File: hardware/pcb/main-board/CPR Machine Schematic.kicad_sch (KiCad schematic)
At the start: 0 parts

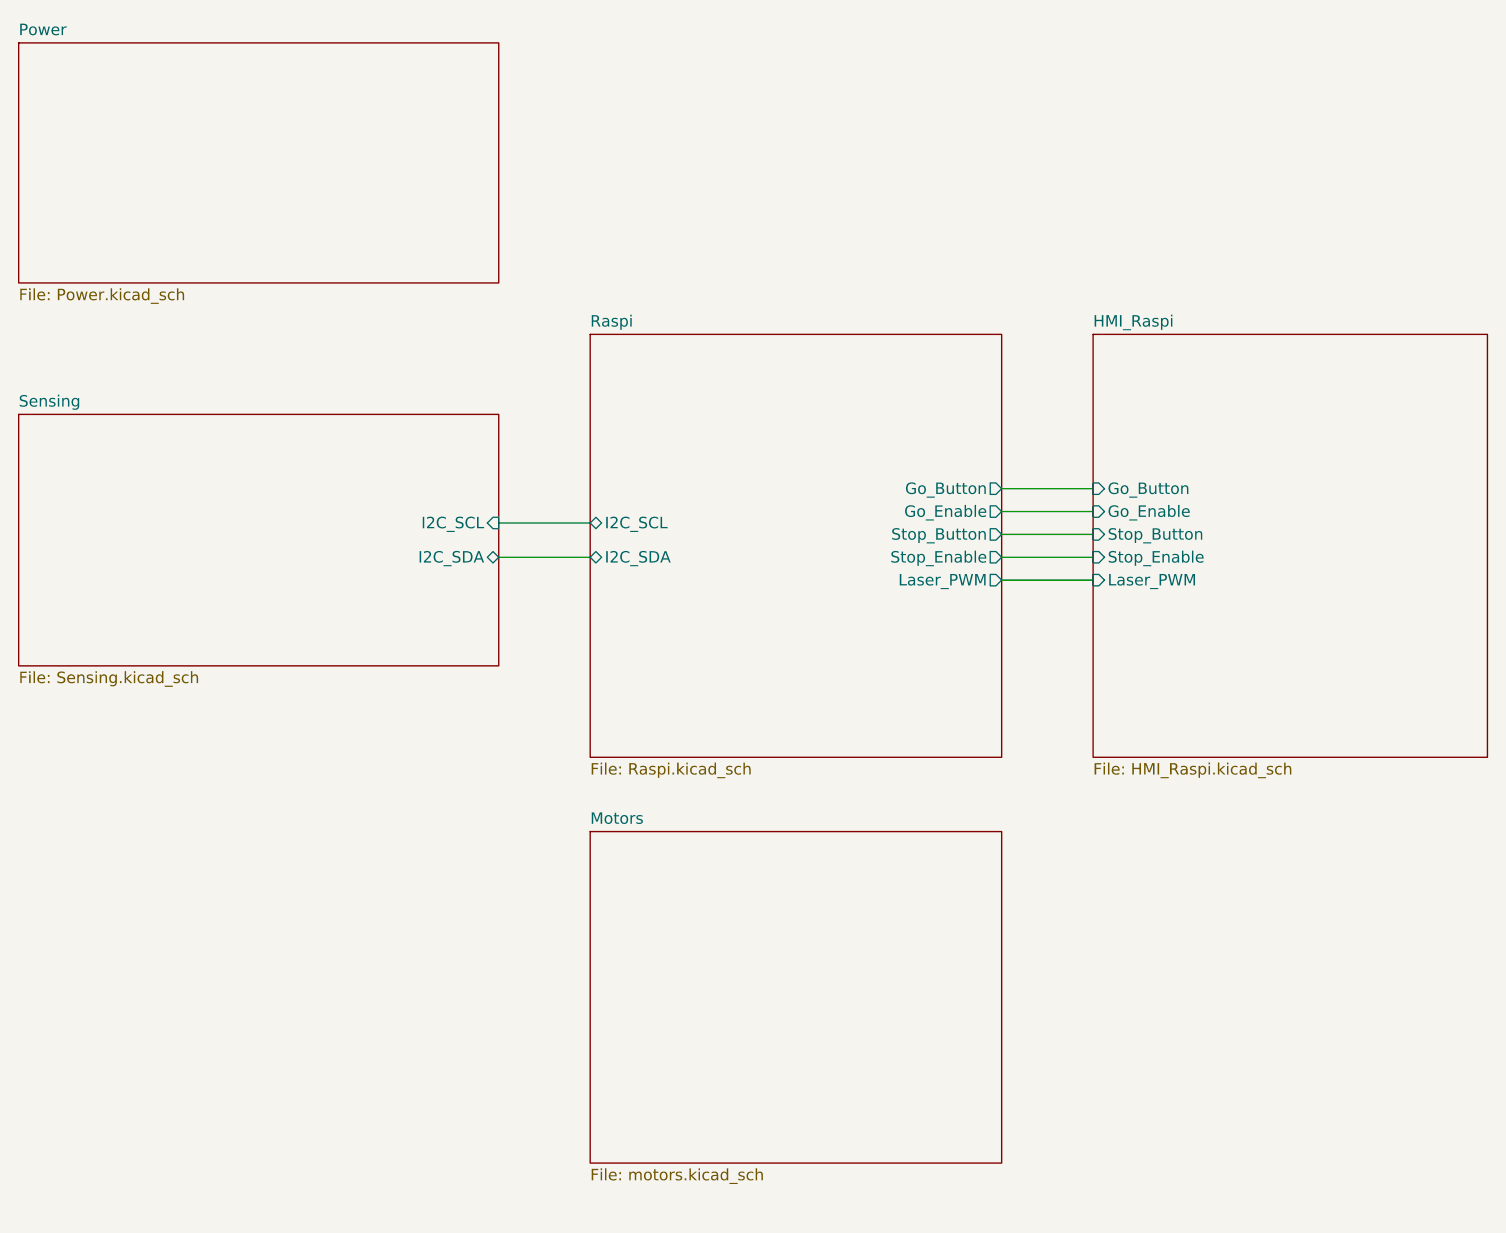
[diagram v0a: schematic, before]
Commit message: Start of CAN-FD
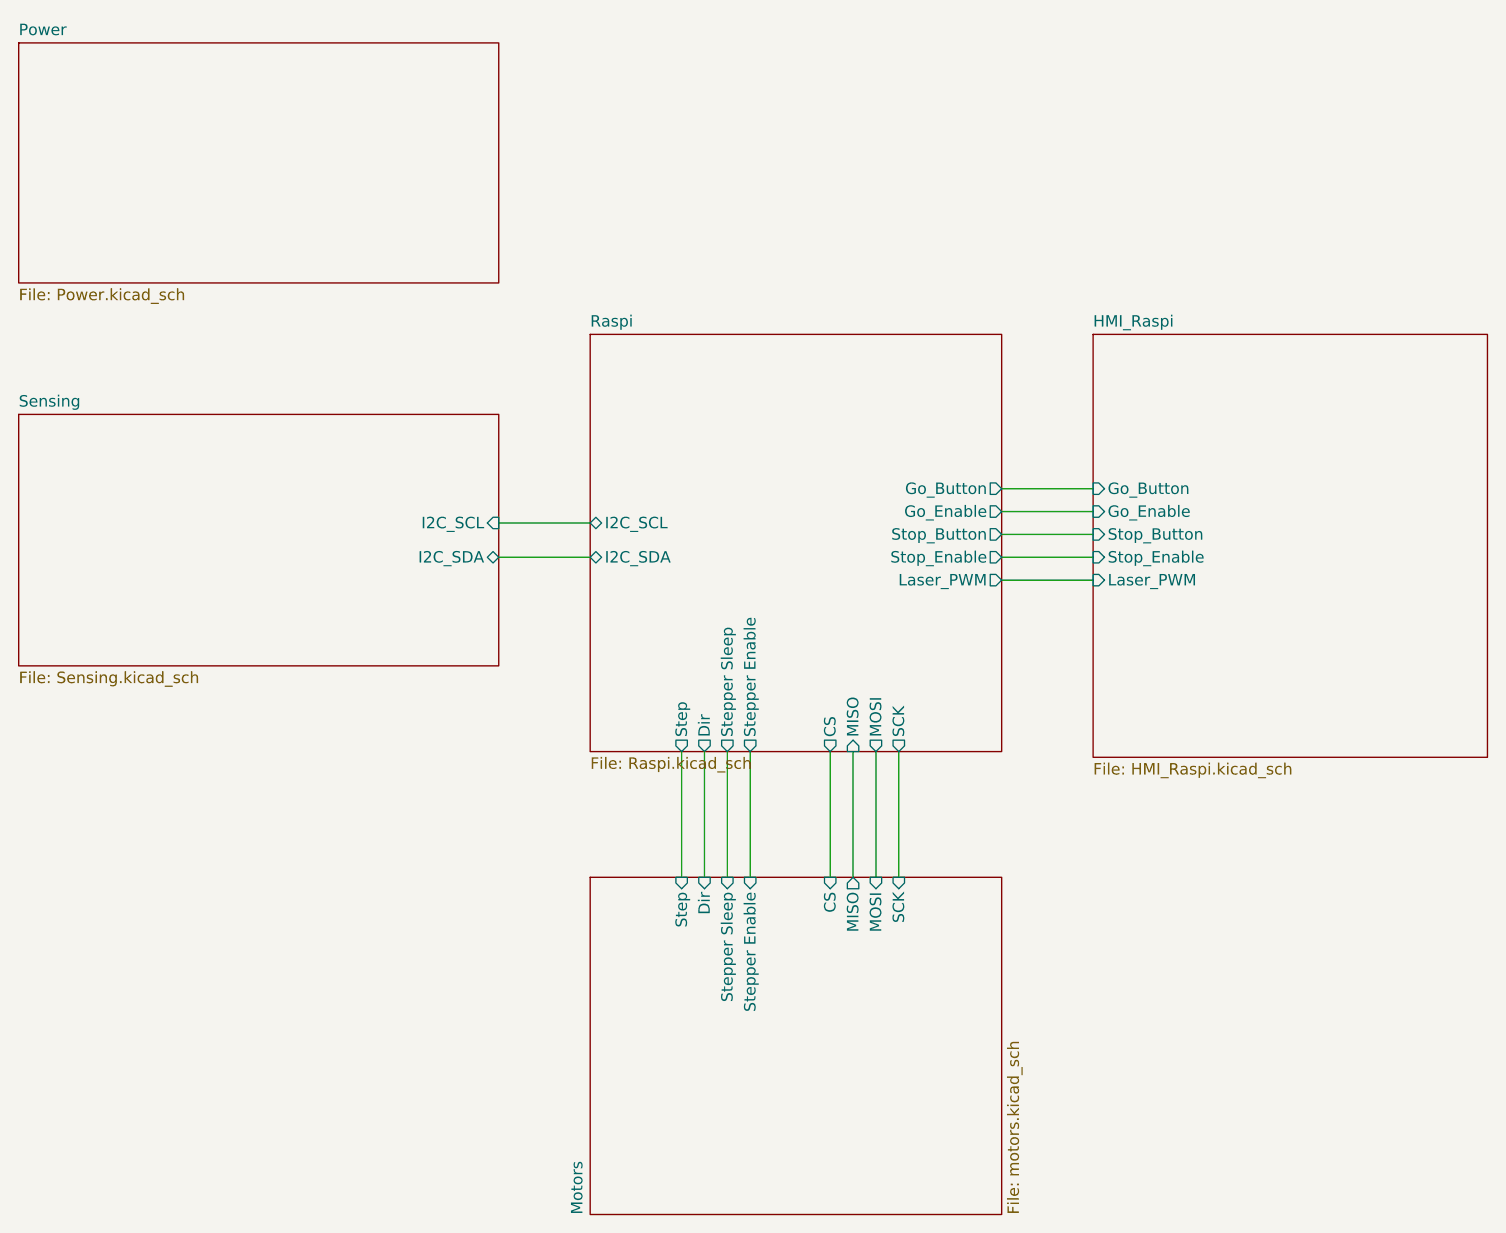
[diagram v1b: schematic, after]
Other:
- sheet Motors ports: added CS, Dir, MISO, MOSI, SCK, Step, Stepper Enable, Stepper Sleep; removed none
- sheet Raspi ports: added CS, Dir, MISO, MOSI, SCK, Step, Stepper Enable, Stepper Sleep; removed none
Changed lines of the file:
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@@
+	(wire
+		(pts
+			(xy 138.43 105.41) (xy 138.43 119.38)
+		)
+		(stroke
+			(width 0)
+			(type default)
+		)
+	)
 	(wire
 		(pts
@@
 	(wire
 		(pts
+			(xy 133.35 105.41) (xy 133.35 119.38)
+		)
+		(stroke
+			(width 0)
+			(type default)
+		)
+	)
+	(wire
+		(pts
+			(xy 130.81 105.41) (xy 130.81 119.38)
+		)
+		(stroke
+			(width 0)
+			(type default)
+		)
+	)
+	(wire
+		(pts
+			(xy 152.4 105.41) (xy 152.4 119.38)
+		)
+		(stroke
+			(width 0)
+			(type default)
+		)
+	)
+	(wire
+		(pts
+			(xy 147.32 105.41) (xy 147.32 119.38)
+		)
+		(stroke
+			(width 0)
+			(type default)
+		)
+	)
+	(wire
+		(pts
+			(xy 135.89 105.41) (xy 135.89 119.38)
+		)
+		(stroke
+			(width 0)
+			(type default)
+		)
+	)
+	(wire
+		(pts
 			(xy 166.37 83.82) (xy 176.53 83.82)
 		)
@@
 	(wire
 		(pts
+			(xy 154.94 105.41) (xy 154.94 119.38)
+		)
+		(stroke
+			(width 0)
+			(type default)
+		)
+	)
+	(wire
+		(pts
 			(xy 110.49 80.01) (xy 120.65 80.01)
 		)
@@
 		(pts
 			(xy 166.37 78.74) (xy 176.53 78.74)
+		)
+		(stroke
+			(width 0)
+			(type default)
+		)
+	)
+	(wire
+		(pts
+			(xy 149.86 105.41) (xy 149.86 119.38)
 		)
 		(stroke
@@
 	(sheet
 		(at 120.65 59.055)
-		(size 45.72 46.99)
+		(size 45.72 46.355)
 		(exclude_from_sim no)
 		(in_bom yes)
@@
 		)
 		(property "Sheetfile" "Raspi.kicad_sch"
-			(at 120.65 106.6296 0)
+			(at 120.65 105.9946 0)
 			(show_name no)
 			(do_not_autoplace no)
@@
 				)
 				(justify right)
+			)
+		)
+		(pin "Dir" output
+			(at 133.35 105.41 270)
+			(effects
+				(font
+					(size 1.27 1.27)
+				)
+				(justify left)
+			)
+		)
+		(pin "Step" output
+			(at 130.81 105.41 270)
+			(effects
+				(font
+					(size 1.27 1.27)
+				)
+				(justify left)
+			)
+		)
+		(pin "Stepper Enable" output
+			(at 138.43 105.41 270)
+			(effects
+				(font
+					(size 1.27 1.27)
+				)
+				(justify left)
+			)
+		)
+		(pin "Stepper Sleep" output
+			(at 135.89 105.41 270)
+			(effects
+				(font
+					(size 1.27 1.27)
+				)
+				(justify left)
+			)
+		)
+		(pin "MISO" input
+			(at 149.86 105.41 270)
+			(effects
+				(font
+					(size 1.27 1.27)
+				)
+				(justify left)
+			)
+		)
+		(pin "MOSI" output
+			(at 152.4 105.41 270)
+			(effects
+				(font
+					(size 1.27 1.27)
+				)
+				(justify left)
+			)
+		)
+		(pin "SCK" output
+			(at 154.94 105.41 270)
+			(effects
+				(font
+					(size 1.27 1.27)
+				)
+				(justify left)
+			)
+		)
+		(pin "CS" output
+			(at 147.32 105.41 270)
+			(effects
+				(font
+					(size 1.27 1.27)
+				)
+				(justify left)
 			)
 		)
@@
 	)
 	(sheet
-		(at 120.65 114.3)
-		(size 45.72 36.83)
+		(at 120.65 119.38)
+		(size 45.72 37.465)
 		(exclude_from_sim no)
 		(in_bom yes)
@@
 		)
 		(property "Sheetname" "Motors"
-			(at 120.65 113.5884 0)
+			(at 119.9384 156.845 90)
 			(show_name no)
 			(do_not_autoplace no)
@@
 		)
 		(property "Sheetfile" "motors.kicad_sch"
-			(at 120.65 151.7146 0)
+			(at 166.9546 156.845 90)
 			(show_name no)
 			(do_not_autoplace no)
@@
 			)
 		)
+		(pin "Step" input
+			(at 130.81 119.38 90)
+			(effects
+				(font
+					(size 1.27 1.27)
+				)
+				(justify right)
+			)
+		)
+		(pin "Stepper Sleep" input
+			(at 135.89 119.38 90)
+			(effects
+				(font
+					(size 1.27 1.27)
+				)
+				(justify right)
+			)
+		)
+		(pin "Dir" input
+			(at 133.35 119.38 90)
+			(effects
+				(font
+					(size 1.27 1.27)
+				)
+				(justify right)
+			)
+		)
+		(pin "Stepper Enable" input
+			(at 138.43 119.38 90)
+			(effects
+				(font
+					(size 1.27 1.27)
+				)
+				(justify right)
+			)
+		)
+		(pin "CS" input
+			(at 147.32 119.38 90)
+			(effects
+				(font
+					(size 1.27 1.27)
+				)
+				(justify right)
+			)
+		)
+		(pin "MISO" output
+			(at 149.86 119.38 90)
+			(effects
+				(font
+					(size 1.27 1.27)
+				)
+				(justify right)
+			)
+		)
+		(pin "MOSI" input
+			(at 152.4 119.38 90)
+			(effects
+				(font
+					(size 1.27 1.27)
+				)
+				(justify right)
+			)
+		)
+		(pin "SCK" input
+			(at 154.94 119.38 90)
+			(effects
+				(font
+					(size 1.27 1.27)
+				)
+				(justify right)
+			)
+		)

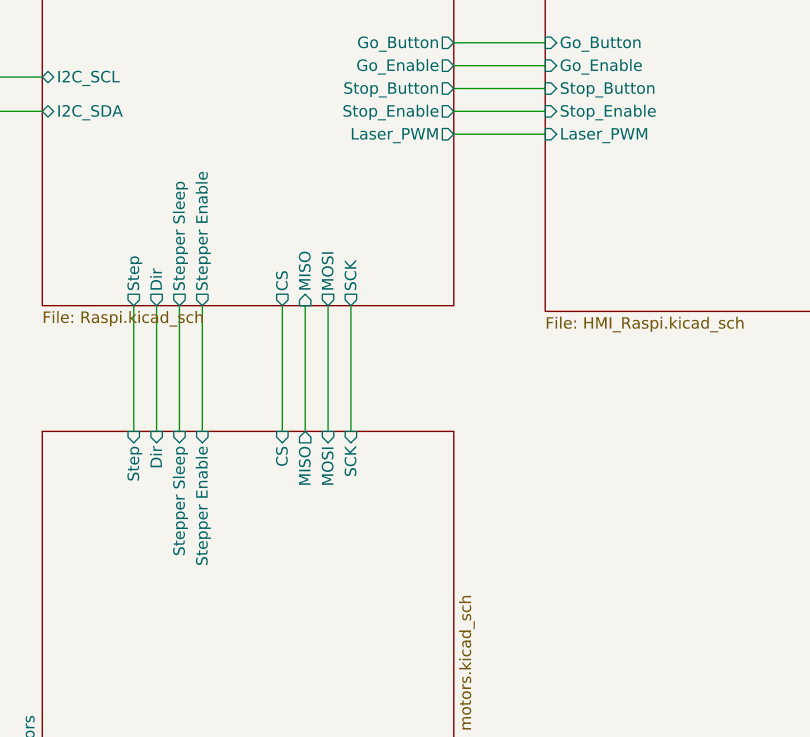
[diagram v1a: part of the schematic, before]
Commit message: CAN-FD Transceiver Done
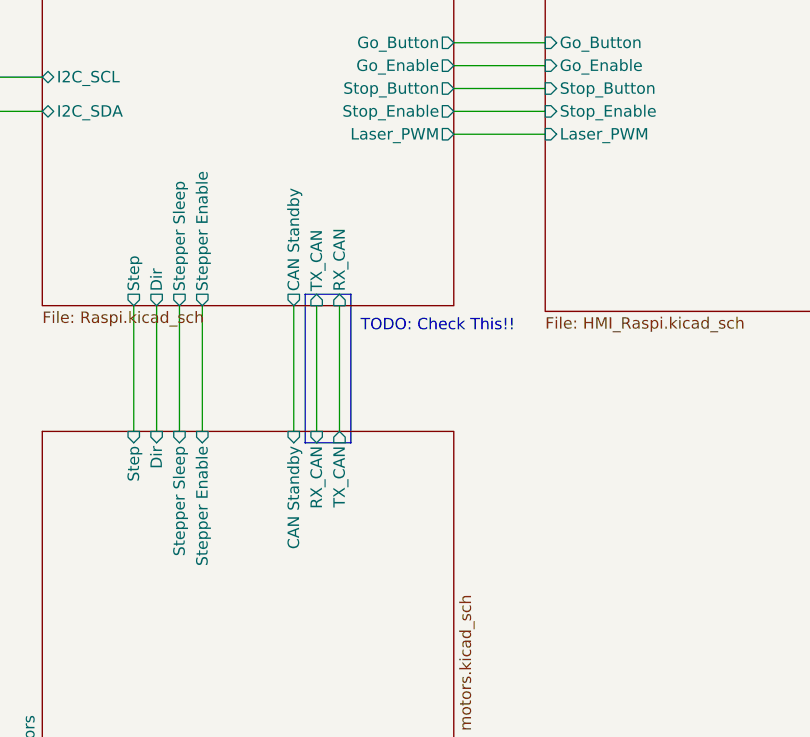
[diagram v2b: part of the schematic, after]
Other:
- sheet Motors ports: added CAN Standby, RX_CAN, TX_CAN; removed CS, MISO, MOSI, SCK
- sheet Raspi ports: added CAN Standby, RX_CAN, TX_CAN; removed CS, MISO, MOSI, SCK
- note added: "TODO: Check This!!"
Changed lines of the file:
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@@
 	(generator_version "10.0")
 	(paper "A4")
+	(rectangle
+		(start 149.86 104.14)
+		(end 154.94 120.65)
+		(stroke
+			(width 0)
+			(type default)
+		)
+		(fill
+			(type none)
+		)
+	)
+	(text "TODO: Check This!!"
+		(exclude_from_sim no)
+		(at 164.592 107.696 0)
+		(effects
+			(font
+				(size 1.27 1.27)
+			)
+		)
+	)
 	(wire
 		(pts
@@
 	(wire
 		(pts
-			(xy 152.4 105.41) (xy 152.4 119.38)
-		)
-		(stroke
-			(width 0)
-			(type default)
-		)
-	)
-	(wire
-		(pts
-			(xy 147.32 105.41) (xy 147.32 119.38)
+			(xy 151.13 105.41) (xy 151.13 119.38)
+		)
+		(stroke
+			(width 0)
+			(type default)
+		)
+	)
+	(wire
+		(pts
+			(xy 148.59 105.41) (xy 148.59 119.38)
+		)
+		(stroke
+			(width 0)
+			(type default)
+		)
+	)
+	(wire
+		(pts
+			(xy 153.67 105.41) (xy 153.67 119.38)
 		)
 		(stroke
@@
 	(wire
 		(pts
-			(xy 154.94 105.41) (xy 154.94 119.38)
-		)
-		(stroke
-			(width 0)
-			(type default)
-		)
-	)
-	(wire
-		(pts
 			(xy 110.49 80.01) (xy 120.65 80.01)
 		)
@@
 		(pts
 			(xy 166.37 78.74) (xy 176.53 78.74)
-		)
-		(stroke
-			(width 0)
-			(type default)
-		)
-	)
-	(wire
-		(pts
-			(xy 149.86 105.41) (xy 149.86 119.38)
 		)
 		(stroke
@@
 			)
 		)
-		(pin "MISO" input
-			(at 149.86 105.41 270)
-			(effects
-				(font
-					(size 1.27 1.27)
-				)
-				(justify left)
-			)
-		)
-		(pin "MOSI" output
-			(at 152.4 105.41 270)
-			(effects
-				(font
-					(size 1.27 1.27)
-				)
-				(justify left)
-			)
-		)
-		(pin "SCK" output
-			(at 154.94 105.41 270)
-			(effects
-				(font
-					(size 1.27 1.27)
-				)
-				(justify left)
-			)
-		)
-		(pin "CS" output
-			(at 147.32 105.41 270)
+		(pin "CAN Standby" output
+			(at 148.59 105.41 270)
+			(effects
+				(font
+					(size 1.27 1.27)
+				)
+				(justify left)
+			)
+		)
+		(pin "RX_CAN" input
+			(at 153.67 105.41 270)
+			(effects
+				(font
+					(size 1.27 1.27)
+				)
+				(justify left)
+			)
+		)
+		(pin "TX_CAN" input
+			(at 151.13 105.41 270)
 			(effects
 				(font
@@
 			)
 		)
-		(pin "CS" input
-			(at 147.32 119.38 90)
-			(effects
-				(font
-					(size 1.27 1.27)
-				)
-				(justify right)
-			)
-		)
-		(pin "MISO" output
-			(at 149.86 119.38 90)
-			(effects
-				(font
-					(size 1.27 1.27)
-				)
-				(justify right)
-			)
-		)
-		(pin "MOSI" input
-			(at 152.4 119.38 90)
-			(effects
-				(font
-					(size 1.27 1.27)
-				)
-				(justify right)
-			)
-		)
-		(pin "SCK" input
-			(at 154.94 119.38 90)
-			(effects
-				(font
+		(pin "CAN Standby" input
+			(at 148.59 119.38 90)
+			(effects
+				(font
+					(size 1.27 1.27)
+				)
+				(justify right)
+			)
+		)
+		(pin "RX_CAN" input
+			(at 151.13 119.38 90)
+			(effects
+				(font
+					(size 1.27 1.27)
+				)
+				(justify right)
+			)
+		)
+		(pin "TX_CAN" output
+			(at 153.67 119.38 90)
+			(effects
+				(font
